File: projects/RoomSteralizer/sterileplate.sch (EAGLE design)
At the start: 11 parts, among them J2 POWER_JACKPTH_LOCK, Q1 Transistor >= 1.5Amp

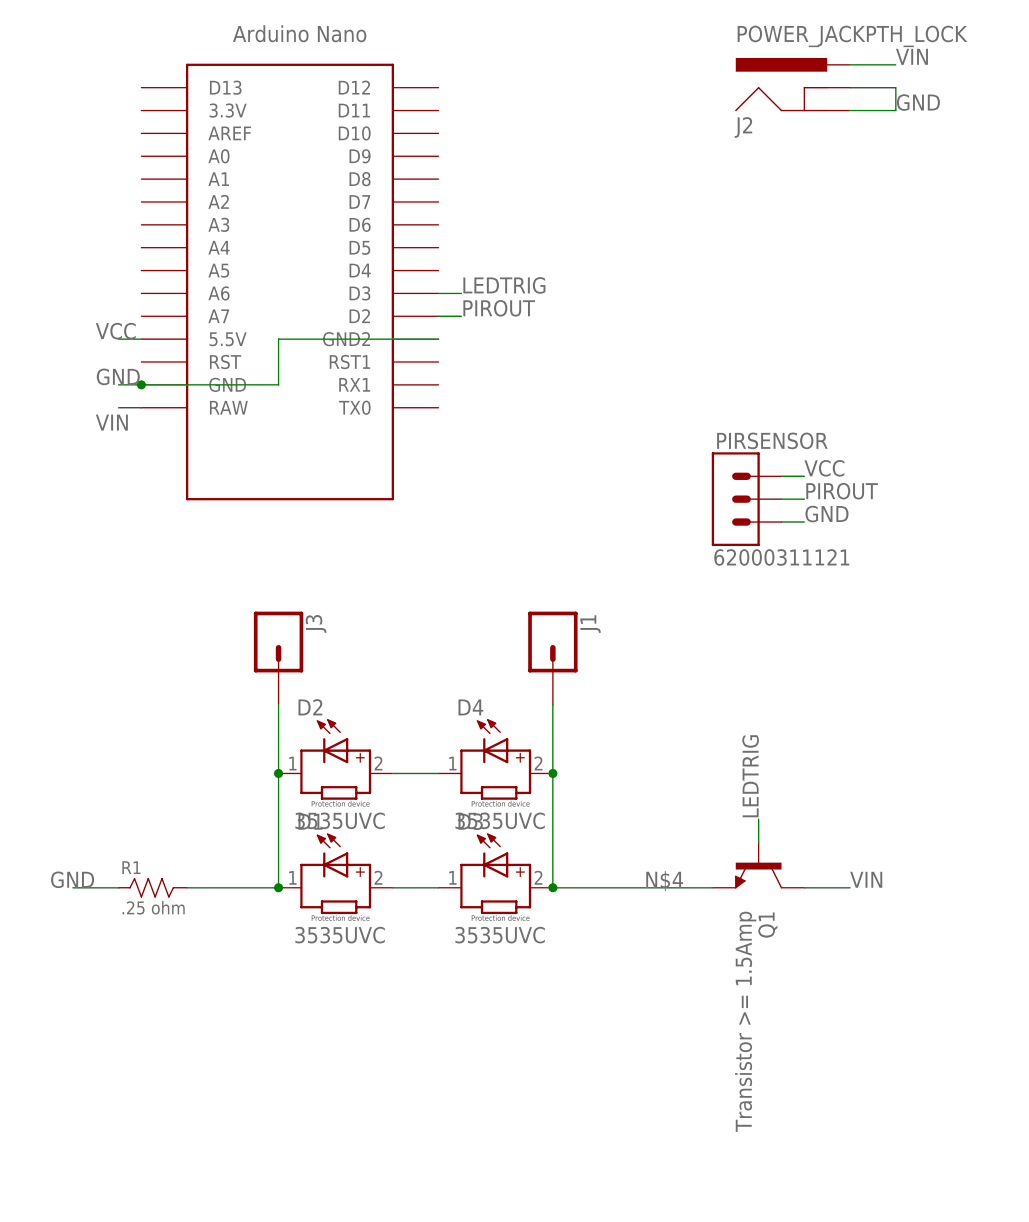
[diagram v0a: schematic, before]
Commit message: asd
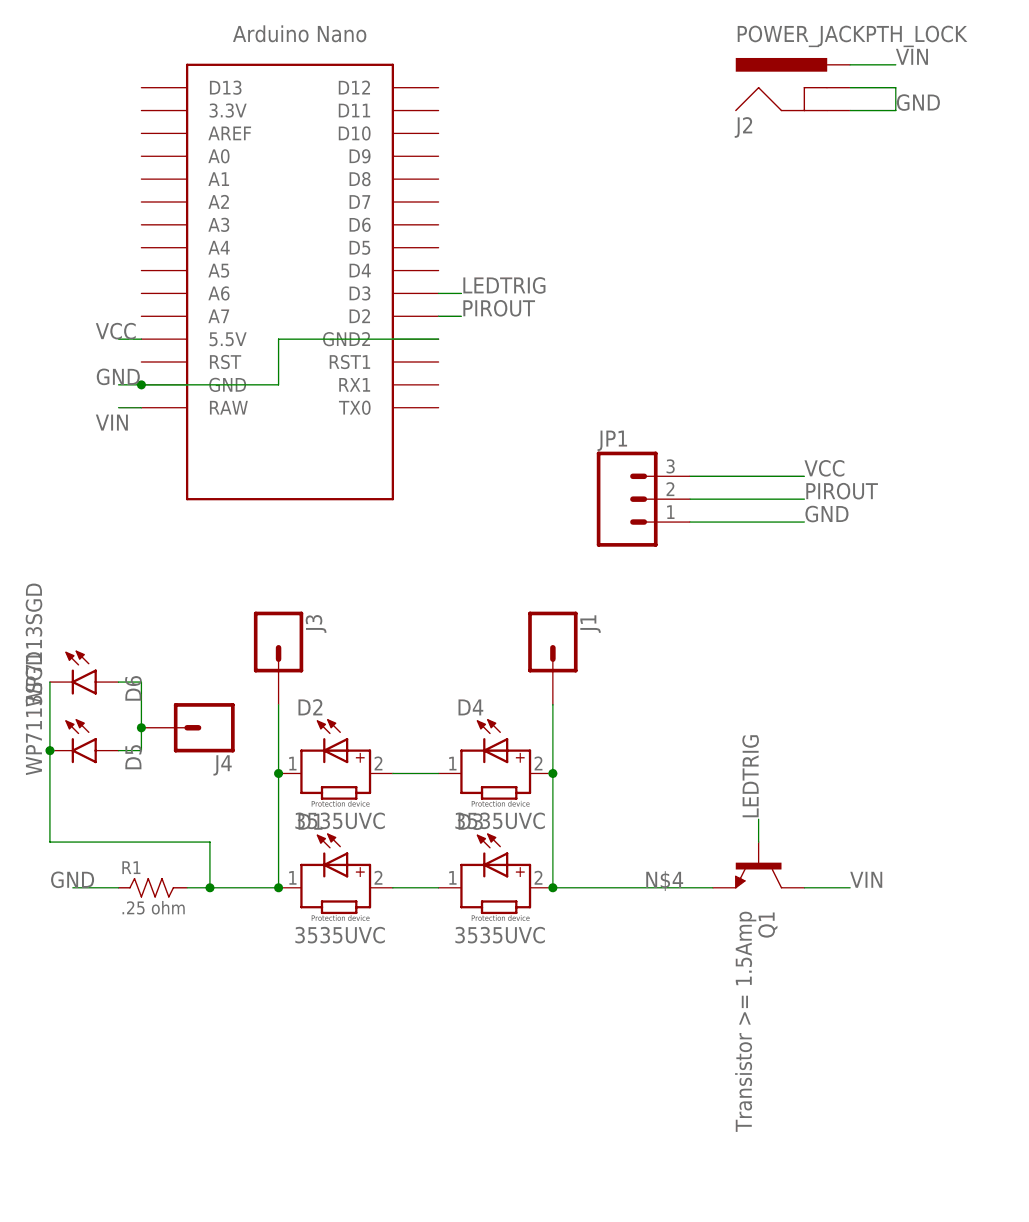
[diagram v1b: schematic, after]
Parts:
- removed PIRSENSOR: 62000311121, Headers:62000311121
- added D5, D6: WP7113SGD, LED:WP7113SGD
- added J4: (no value), SparkFun-Connectors:CONN_01PTH_2MM
- added JP1: (no value), SparkFun:M03PTH
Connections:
- removed net N$3: D1.1, D2.1, J3.1, R1.2
- new net N$6: D5.A, D6.A, J4.1
- new net N$7: D1.1, D2.1, D5.C, D6.C, J3.1, R1.2
- net GND: now also JP1.1; no longer PIRSENSOR.3
- net PIROUT: now also JP1.2; no longer PIRSENSOR.2
- net VCC: now also JP1.3; no longer PIRSENSOR.1
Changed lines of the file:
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@@
-<attribute name="OC_NEWARK" value="unknown"/>
-</part>
-<part name="PIRSENSOR" library="Headers" library_urn="urn:adsk.eagle:library:11687645" deviceset="62000311121" device="" package3d_urn="urn:adsk.eagle:package:11432193/2">
-<attribute name="MF" value=""/>
-<attribute name="MPN" value=""/>
 <attribute name="OC_NEWARK" value="unknown"/>
 </part>
@@
 <part name="J1" library="SparkFun-Connectors" deviceset="CONN_01" device="PTH_2MM"/>
 <part name="J3" library="SparkFun-Connectors" deviceset="CONN_01" device="PTH_2MM"/>
+<part name="JP1" library="SparkFun" deviceset="M03" device="PTH"/>
+<part name="D5" library="LED" library_urn="urn:adsk.eagle:library:11396303" deviceset="WP7113SGD" device="" package3d_urn="urn:adsk.eagle:package:10893501/2"/>
+<part name="D6" library="LED" library_urn="urn:adsk.eagle:library:11396303" deviceset="WP7113SGD" device="" package3d_urn="urn:adsk.eagle:package:10893501/2"/>
+<part name="J4" library="SparkFun-Connectors" deviceset="CONN_01" device="PTH_2MM"/>
 </parts>
 <sheets>
@@
 <attribute name="MPN" x="38.1" y="60.96" size="1.778" layer="96" display="off"/>
 </instance>
-<instance part="PIRSENSOR" gate="G$1" x="81.28" y="30.48" smashed="yes">
-<attribute name="NAME" x="78.994" y="36.068" size="1.778" layer="95"/>
-<attribute name="VALUE" x="78.74" y="23.114" size="1.778" layer="96"/>
-<attribute name="OC_NEWARK" x="81.28" y="30.48" size="1.778" layer="96" display="off"/>
-<attribute name="MF" x="81.28" y="30.48" size="1.778" layer="96" display="off"/>
-</instance>
 <instance part="R1" gate="G$1" x="15.24" y="-12.7" smashed="yes">
 <attribute name="NAME" x="12.954" y="-11.176" size="1.4224" layer="95"/>
@@
 <attribute name="NAME" x="33.528" y="17.78" size="1.778" layer="95" font="vector" rot="R270"/>
 </instance>
+<instance part="JP1" gate="G$1" x="68.58" y="30.48" smashed="yes">
+<attribute name="VALUE" x="66.04" y="22.86" size="1.778" layer="96"/>
+<attribute name="NAME" x="66.04" y="36.322" size="1.778" layer="95"/>
+</instance>
+<instance part="D5" gate="G$1" x="10.16" y="2.54" smashed="yes" rot="R270">
+<attribute name="NAME" x="15.24" y="0.254" size="1.778" layer="95" rot="R90"/>
+<attribute name="VALUE" x="4.191" y="-0.254" size="1.778" layer="96" rot="R90"/>
+</instance>
+<instance part="D6" gate="G$1" x="10.16" y="10.16" smashed="yes" rot="R270">
+<attribute name="NAME" x="15.24" y="7.874" size="1.778" layer="95" rot="R90"/>
+<attribute name="VALUE" x="4.191" y="7.366" size="1.778" layer="96" rot="R90"/>
+</instance>
+<instance part="J4" gate="G$1" x="22.86" y="5.08" smashed="yes" rot="R180">
+<attribute name="VALUE" x="25.4" y="9.906" size="1.778" layer="96" font="vector" rot="R180"/>
+<attribute name="NAME" x="25.4" y="2.032" size="1.778" layer="95" font="vector" rot="R180"/>
+</instance>
 </instances>
 <busses>
@@
 <pinref part="D1" gate="G$1" pin="2"/>
 <wire x1="48.26" y1="-12.7" x2="43.18" y2="-12.7" width="0.1524" layer="91"/>
-</segment>
-</net>
-<net name="N$3" class="0">
-<segment>
-<pinref part="D2" gate="G$1" pin="1"/>
-<pinref part="D1" gate="G$1" pin="1"/>
-<wire x1="30.48" y1="0" x2="30.48" y2="-12.7" width="0.1524" layer="91"/>
-<pinref part="R1" gate="G$1" pin="2"/>
-<wire x1="30.48" y1="-12.7" x2="20.32" y2="-12.7" width="0.1524" layer="91"/>
-<junction x="30.48" y="-12.7"/>
-<pinref part="J3" gate="G$1" pin="1"/>
-<wire x1="30.48" y1="7.62" x2="30.48" y2="0" width="0.1524" layer="91"/>
-<junction x="30.48" y="0"/>
 </segment>
 </net>
@@
 </segment>
 <segment>
-<pinref part="PIRSENSOR" gate="G$1" pin="3"/>
-<wire x1="86.36" y1="27.94" x2="88.9" y2="27.94" width="0.1524" layer="91"/>
 <label x="88.9" y="27.94" size="1.778" layer="95"/>
+<pinref part="JP1" gate="G$1" pin="1"/>
+<wire x1="76.2" y1="27.94" x2="88.9" y2="27.94" width="0.1524" layer="91"/>
 </segment>
 </net>
@@
 <net name="PIROUT" class="0">
 <segment>
-<pinref part="PIRSENSOR" gate="G$1" pin="2"/>
-<wire x1="86.36" y1="30.48" x2="88.9" y2="30.48" width="0.1524" layer="91"/>
 <label x="88.9" y="30.48" size="1.778" layer="95"/>
+<pinref part="JP1" gate="G$1" pin="2"/>
+<wire x1="88.9" y1="30.48" x2="76.2" y2="30.48" width="0.1524" layer="91"/>
 </segment>
 <segment>
@@
 <net name="VCC" class="0">
 <segment>
-<pinref part="PIRSENSOR" gate="G$1" pin="1"/>
-<wire x1="86.36" y1="33.02" x2="88.9" y2="33.02" width="0.1524" layer="91"/>
 <label x="88.9" y="33.02" size="1.778" layer="95"/>
+<pinref part="JP1" gate="G$1" pin="3"/>
+<wire x1="76.2" y1="33.02" x2="88.9" y2="33.02" width="0.1524" layer="91"/>
 </segment>
 <segment>
@@
 </segment>
 </net>
+<net name="N$6" class="0">
+<segment>
+<pinref part="D5" gate="G$1" pin="A"/>
+<pinref part="J4" gate="G$1" pin="1"/>
+<wire x1="12.7" y1="2.54" x2="15.24" y2="2.54" width="0.1524" layer="91"/>
+<wire x1="15.24" y1="2.54" x2="15.24" y2="5.08" width="0.1524" layer="91"/>
+<pinref part="D6" gate="G$1" pin="A"/>
+<wire x1="12.7" y1="10.16" x2="15.24" y2="10.16" width="0.1524" layer="91"/>
+<wire x1="15.24" y1="10.16" x2="15.24" y2="5.08" width="0.1524" layer="91"/>
+<junction x="15.24" y="5.08"/>
+</segment>
+</net>
+<net name="N$7" class="0">
+<segment>
+<pinref part="D6" gate="G$1" pin="C"/>
+<pinref part="D5" gate="G$1" pin="C"/>
+<wire x1="5.08" y1="10.16" x2="5.08" y2="2.54" width="0.1524" layer="91"/>
+<wire x1="5.08" y1="2.54" x2="5.08" y2="-7.62" width="0.1524" layer="91"/>
+<junction x="5.08" y="2.54"/>
+<wire x1="5.08" y1="-7.62" x2="22.86" y2="-7.62" width="0.1524" layer="91"/>
+<pinref part="D2" gate="G$1" pin="1"/>
+<pinref part="D1" gate="G$1" pin="1"/>
+<wire x1="30.48" y1="0" x2="30.48" y2="-12.7" width="0.1524" layer="91"/>
+<pinref part="R1" gate="G$1" pin="2"/>
+<wire x1="30.48" y1="-12.7" x2="22.86" y2="-12.7" width="0.1524" layer="91"/>
+<junction x="30.48" y="-12.7"/>
+<pinref part="J3" gate="G$1" pin="1"/>
+<wire x1="22.86" y1="-12.7" x2="20.32" y2="-12.7" width="0.1524" layer="91"/>
+<wire x1="30.48" y1="7.62" x2="30.48" y2="0" width="0.1524" layer="91"/>
+<junction x="30.48" y="0"/>
+<wire x1="22.86" y1="-7.62" x2="22.86" y2="-12.7" width="0.1524" layer="91"/>
+<junction x="22.86" y="-12.7"/>
+</segment>
+</net>
